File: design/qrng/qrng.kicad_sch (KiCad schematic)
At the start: 7 parts

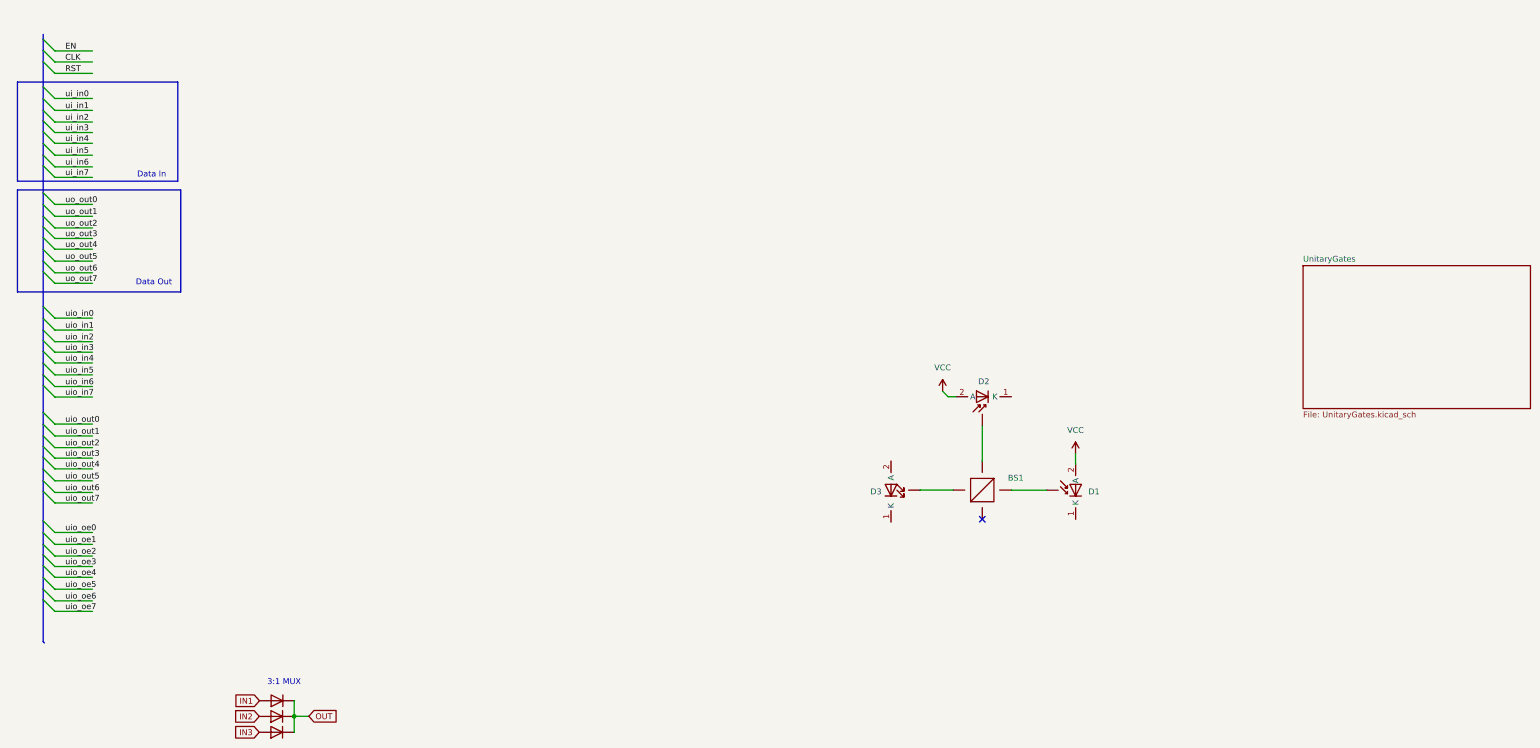
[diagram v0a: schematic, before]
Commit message: Updated KiCAD design
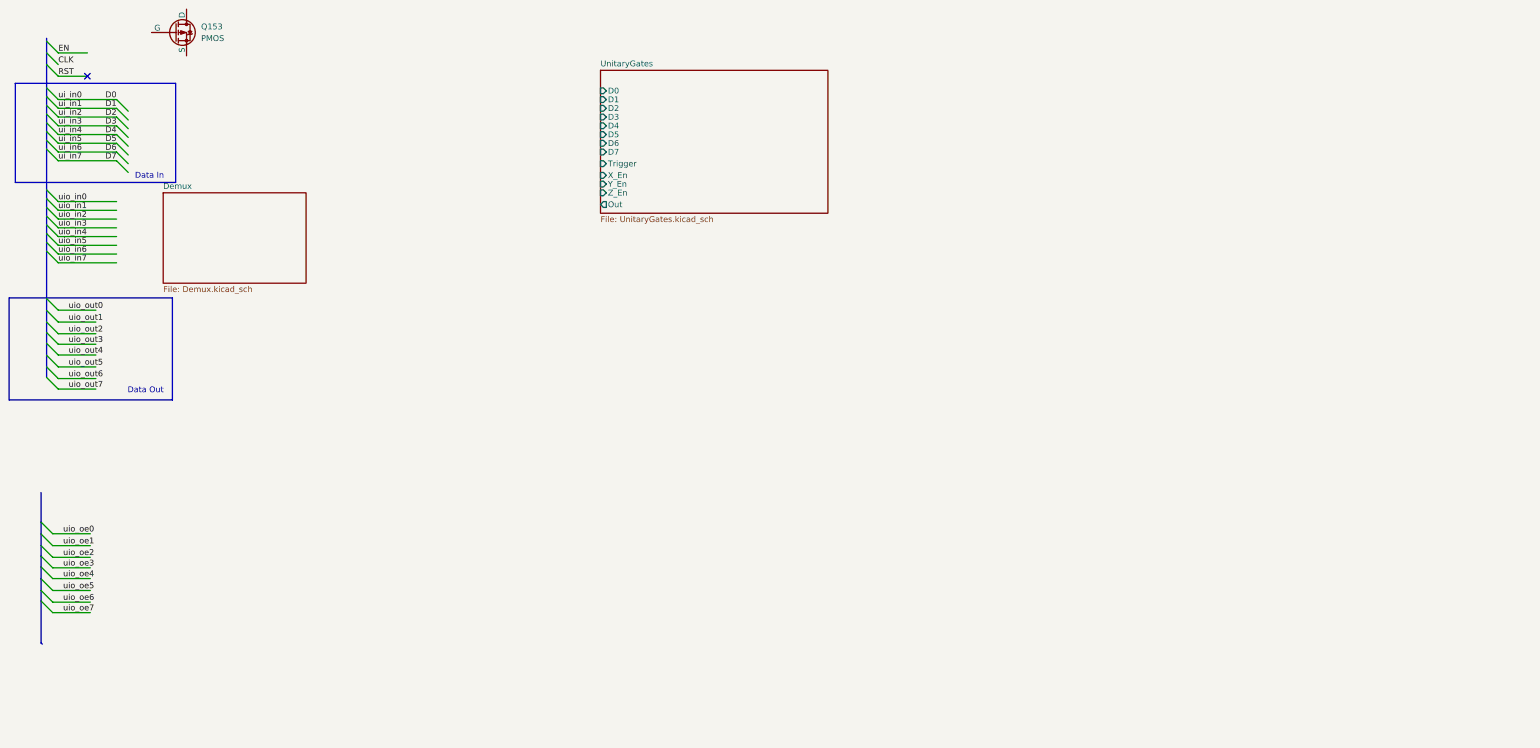
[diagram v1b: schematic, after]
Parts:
- removed BS1: ~, symbol photonic_structures:BeamSplitter
- removed D1, D2: ~, symbol photonic_structures:PhotoDiode
- removed D3: ~, symbol photonic_structures:LED
- removed D4, D5, D6: 1N4001, Diode_THT:D_DO-41_SOD81_P10.16mm_Horizontal, symbol Diode:1N4001
- added Q153: PMOS, symbol Simulation_SPICE:PMOS
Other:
- added sheet Demux (Demux.kicad_sch)
- sheet UnitaryGates ports: added D0, D1, D2, D3, D4, D5, D6, D7, Out, Trigger, X_En, Y_En, Z_En; removed none
- note removed: "3:1 MUX"
